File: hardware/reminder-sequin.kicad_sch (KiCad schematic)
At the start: 32 parts, among them J1 USB_C_Receptacle_USB2.0_16P, J2 uart, J3 swd, SW1 User, SW2 RST, SW3 Vibration_Detect, U1 STM32L011F4Px, U3 CH340N, Y1 32.768kHz

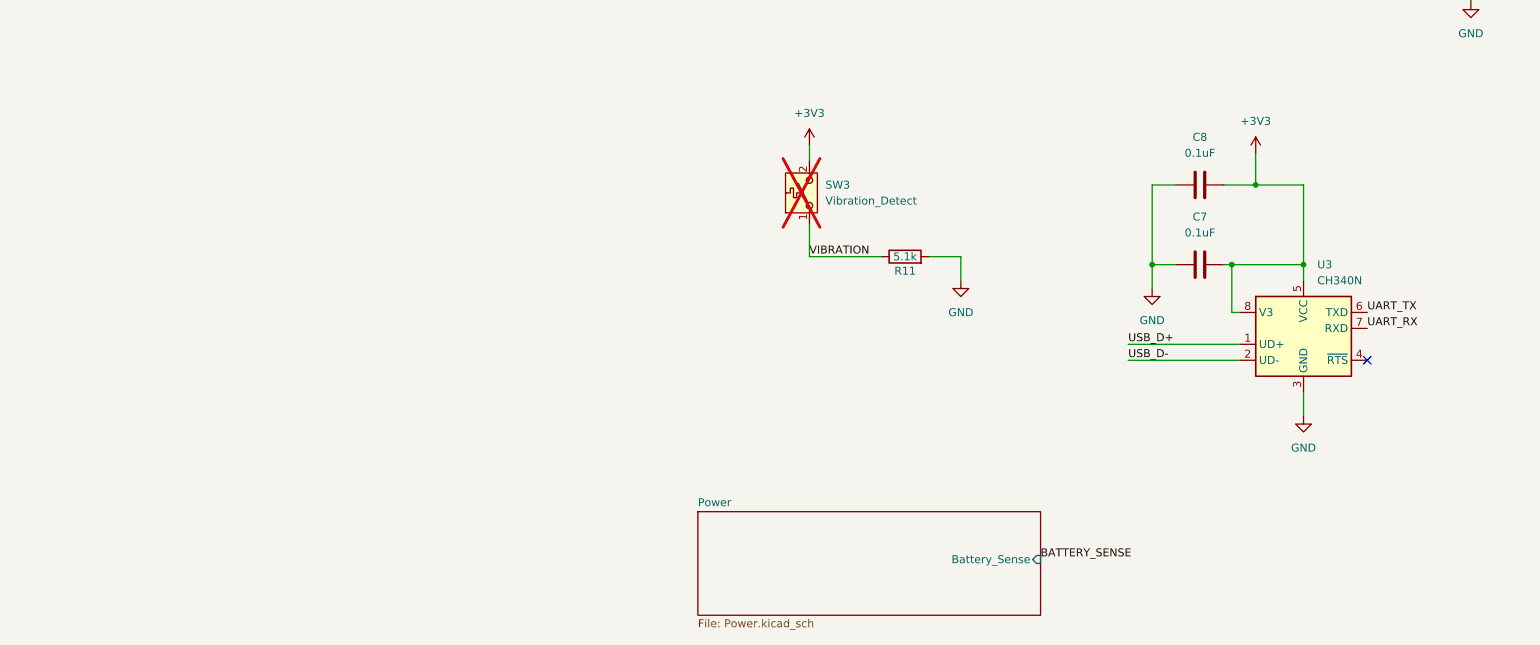
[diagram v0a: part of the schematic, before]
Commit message: bom improvements
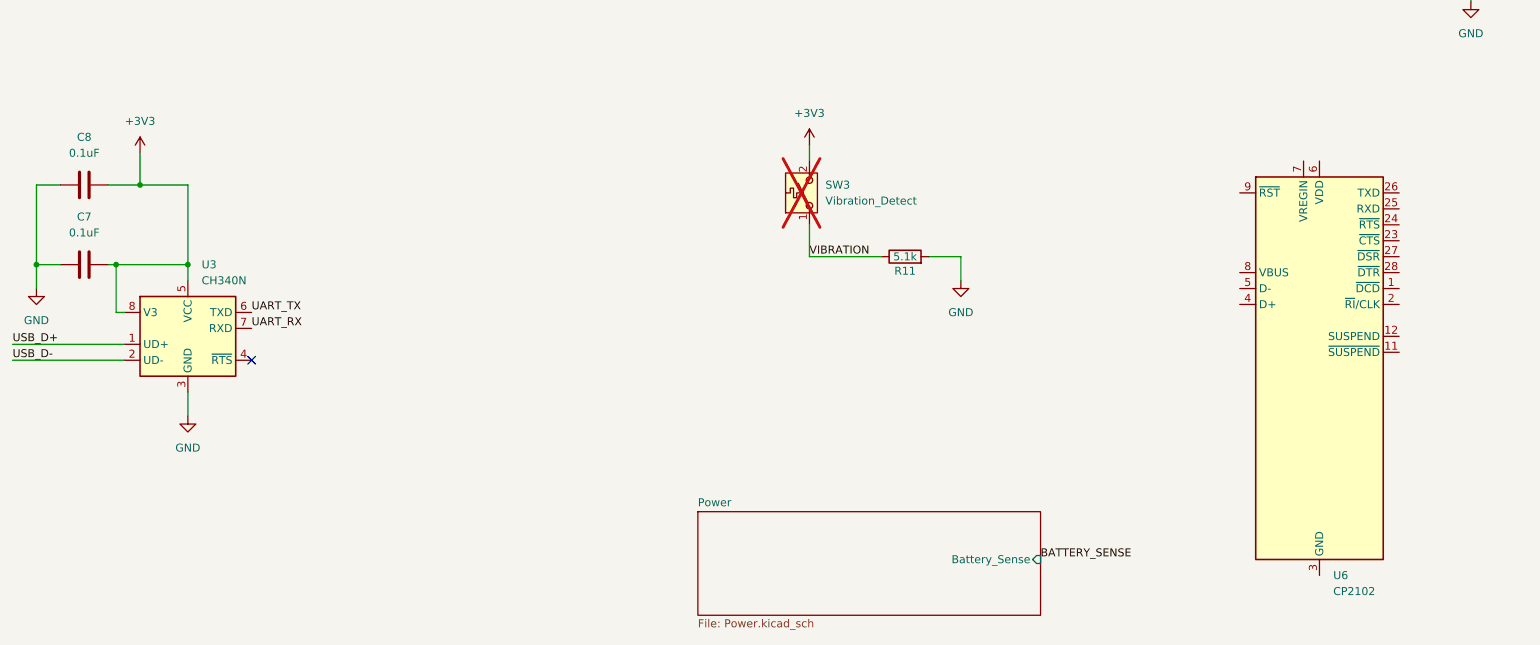
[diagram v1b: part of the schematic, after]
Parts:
- added U6: CP2102, Package_DFN_QFN:QFN-28-1EP_5x5mm_P0.5mm_EP3.35x3.35mm, symbol cat:CP2102
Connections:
- new net: U6.29 (GND), U6.3 (GND)
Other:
- moved on the sheet: C7, C8, U3

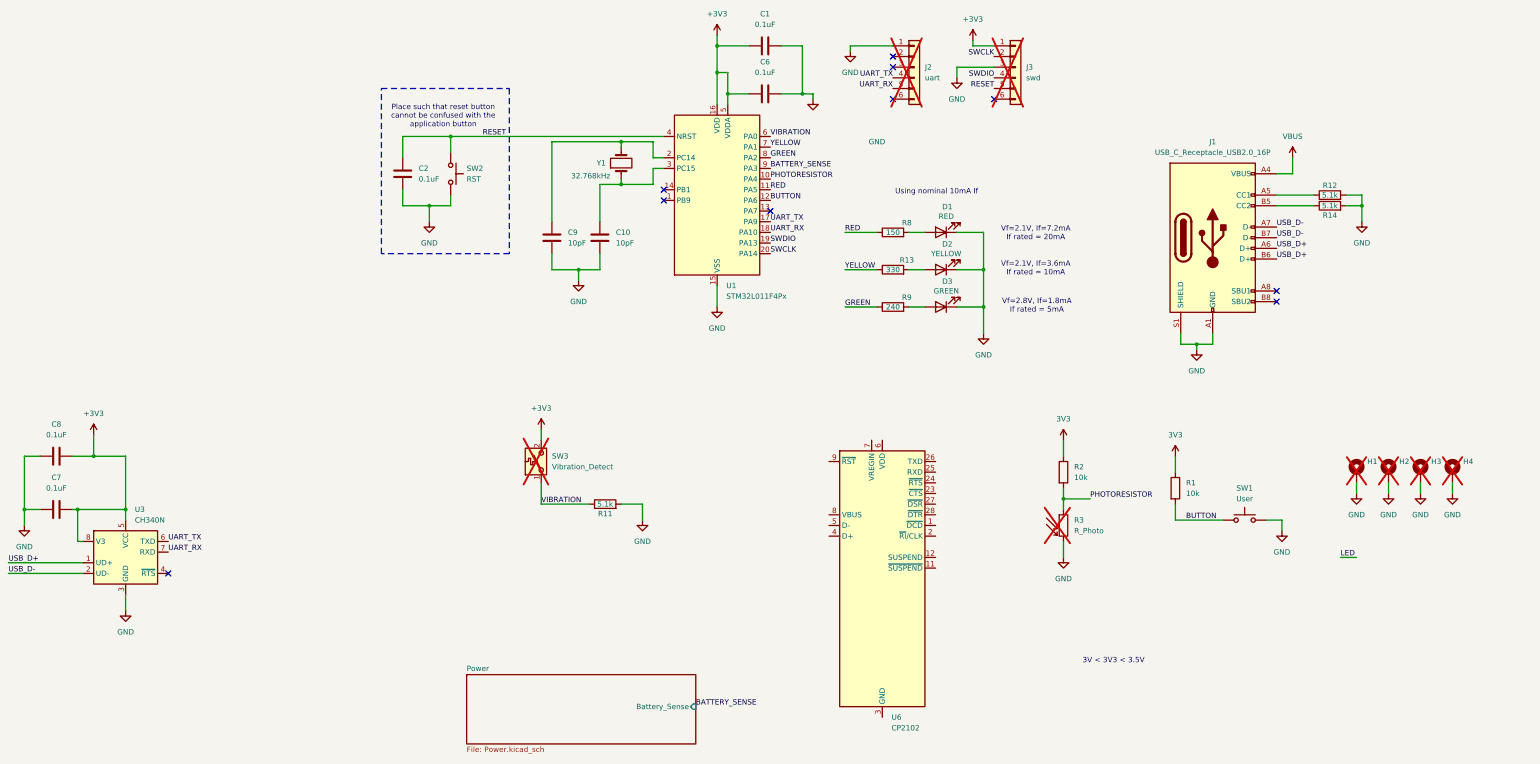
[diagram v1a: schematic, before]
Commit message: switched microcontrollers, again
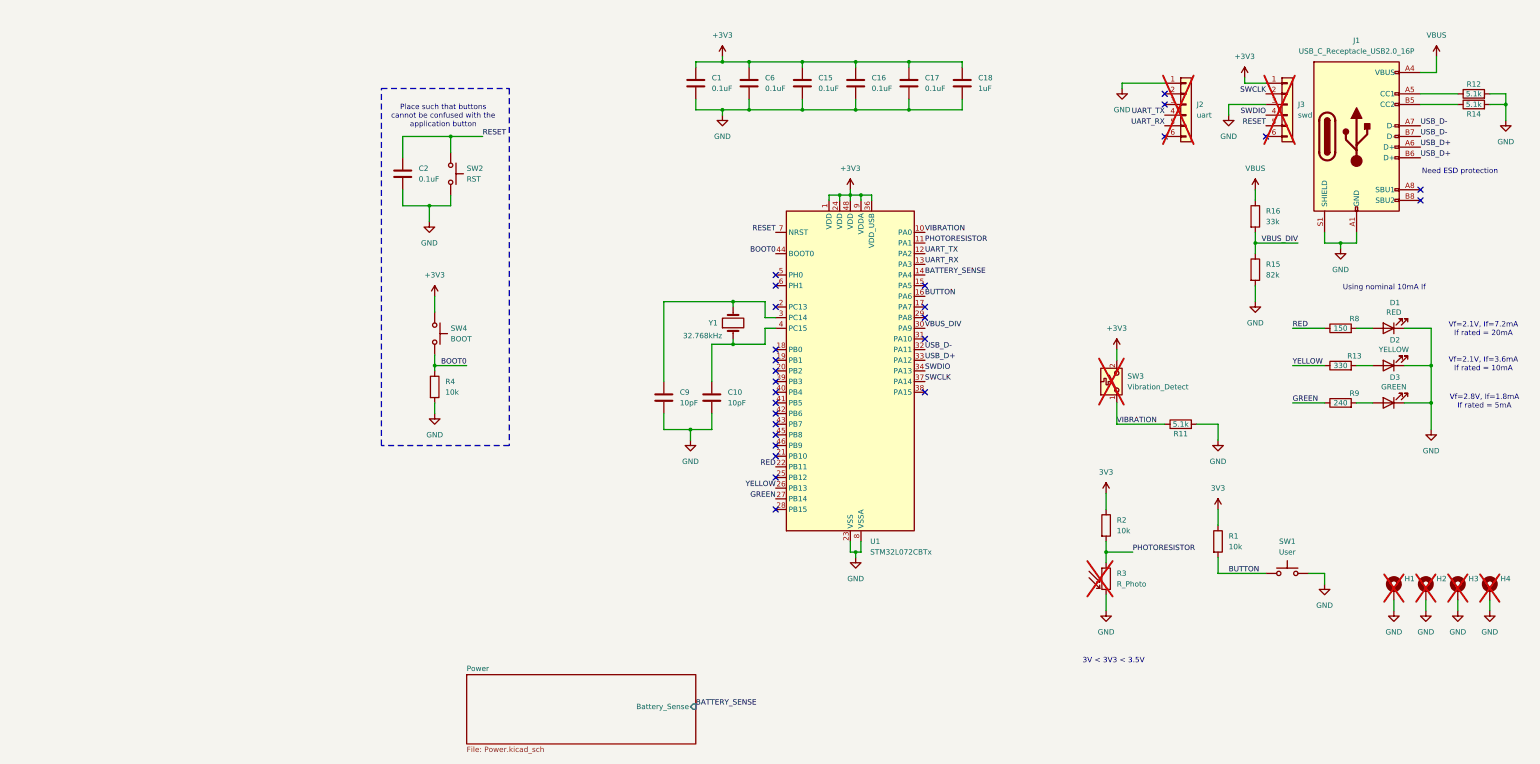
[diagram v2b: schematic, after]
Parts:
- removed C7, C8: 0.1uF, Capacitor_SMD:C_0402_1005Metric, symbol Device:C
- removed U1: STM32L011F4Px, Package_SO:TSSOP-20_4.4x6.5mm_P0.65mm, symbol MCU_ST_STM32L0:STM32L011F4Px
- removed U3: CH340N, Package_SO:SOP-8_3.9x4.9mm_P1.27mm, symbol Interface_USB:CH340N
- removed U6: CP2102, Package_DFN_QFN:QFN-28-1EP_5x5mm_P0.5mm_EP3.35x3.35mm, symbol cat:CP2102
- added C15, C16, C17: 0.1uF, Capacitor_SMD:C_0402_1005Metric, symbol Device:C
- added C18: 1uF, Capacitor_SMD:C_0805_2012Metric, symbol Device:C
- added R15: 82k, Resistor_SMD:R_0603_1608Metric, symbol Device:R
- added R16: 33k, Resistor_SMD:R_0402_1005Metric, symbol Device:R
- added R4: 10k, Resistor_SMD:R_0402_1005Metric, symbol Device:R
- added SW4: BOOT, cat:TS-1088-AR02016, symbol Switch:SW_Push
- added U1: STM32L072CBTx, Package_QFP:LQFP-48_7x7mm_P0.5mm, symbol MCU_ST_STM32L0:STM32L072CBTx
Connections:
- net +3V3: now also C1.2, C6.2, C15.2, C16.2, C17.2, C18.2, SW4.1, U1.1 (VDD), U1.24 (VDD), U1.36 (VDD_USB), U1.48 (VDD), U1.9 (VDDA); no longer C1.1, C6.1
- net BATTERY_SENSE: now also U1.14 (PA4)
- net BUTTON: now also U1.16 (PA6)
- net GND: now also C1.1, C6.1, C15.1, C16.1, C17.1, C18.1, R15.2, R4.2, U1.23 (VSS), U1.35 (VSS), U1.47 (VSS), U1.8 (VSSA); no longer C1.2, C6.2
- net GREEN: now also U1.27 (PB14)
- net PHOTORESISTOR: now also U1.11 (PA1)
- net RED: now also U1.22 (PB11)
- net RESET: now also U1.7 (NRST)
- net SWCLK: now also U1.37 (PA14)
- net SWDIO: now also U1.34 (PA13)
- net UART_RX: now also U1.13 (PA3)
- net UART_TX: now also U1.12 (PA2)
- net USB_D+: now also U1.33 (PA12)
- net USB_D-: now also U1.32 (PA11)
- net VBUS: now also R16.1
- net VIBRATION: now also U1.10 (PA0)
- net YELLOW: now also U1.26 (PB13)
- net at C10.1, Y1.1: now also U1.4 (PC15)
- net at C9.1, Y1.2: now also U1.3 (PC14)
- new net BOOT0: R4.1, SW4.2, U1.44 (BOOT0)
- new net VBUS_DIV: R15.1, R16.2, U1.30 (PA9)
- no-connect marks 10 -> 27
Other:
- note added: "Need ESD protection"
- note added: "Place such that buttons cannot be confused with the application button"
- note removed: "Place such that reset button cannot be confused with the application button"
- moved on the sheet: C1, C10, C6, C9, D1, D2, D3, H1, H2, H3, H4, J1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
